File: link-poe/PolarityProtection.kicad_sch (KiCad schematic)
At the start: 6 parts, among them Q301 BSC010N04LS, Q302 BSC010N04LS, U301 LM74502-Q1

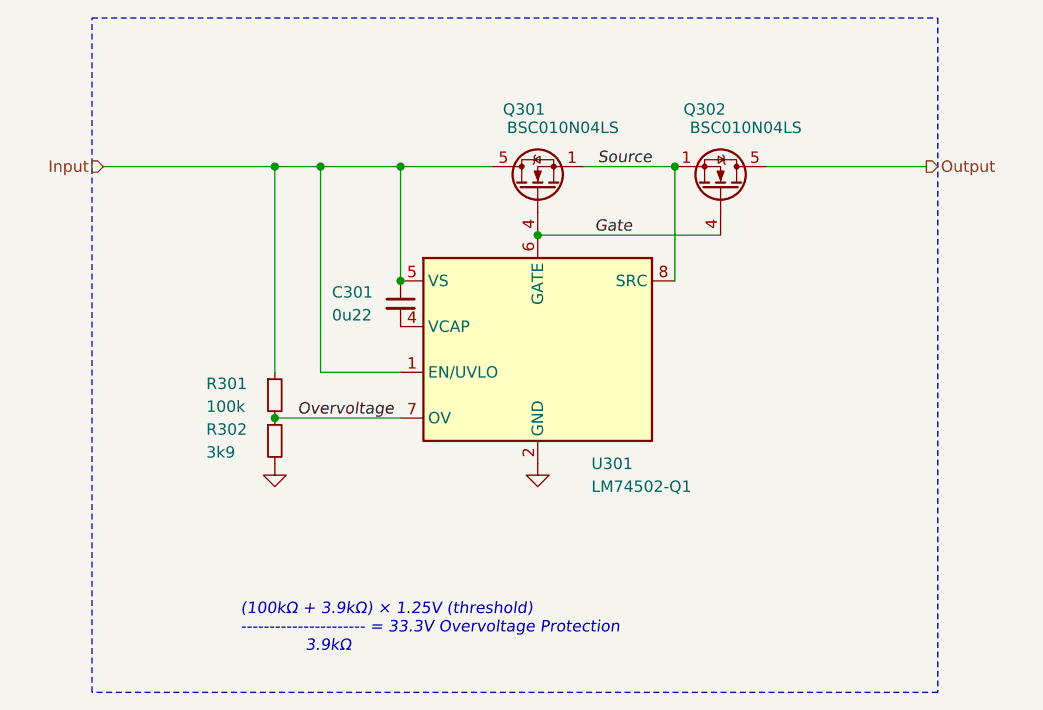
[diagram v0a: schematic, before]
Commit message: Update
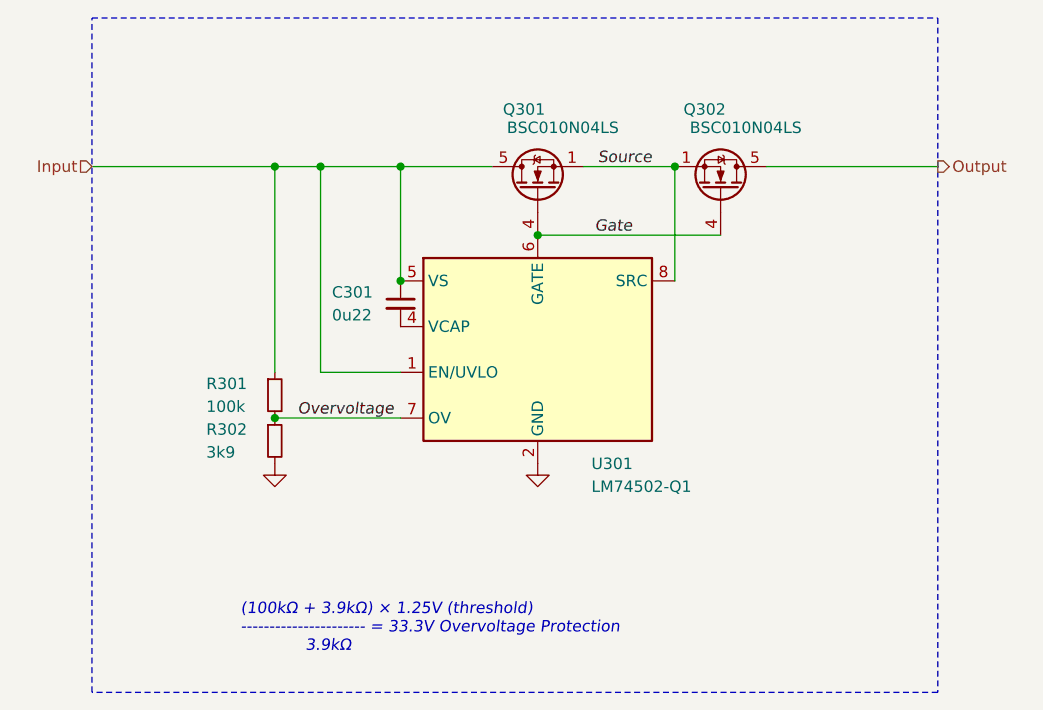
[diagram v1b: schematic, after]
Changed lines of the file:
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@@
 	(wire
 		(pts
-			(xy 102.87 86.36) (xy 121.92 86.36)
+			(xy 101.6 86.36) (xy 121.92 86.36)
 		)
 		(stroke
@@
 	(wire
 		(pts
-			(xy 176.53 86.36) (xy 194.31 86.36)
+			(xy 176.53 86.36) (xy 195.58 86.36)
 		)
 		(stroke
@@
 	(hierarchical_label "Input"
 		(shape input)
-		(at 102.87 86.36 180)
+		(at 101.6 86.36 180)
 		(effects
 			(font
@@
 	(hierarchical_label "Output"
 		(shape output)
-		(at 194.31 86.36 0)
+		(at 195.58 86.36 0)
 		(effects
 			(font

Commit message: Update usb + link-poe
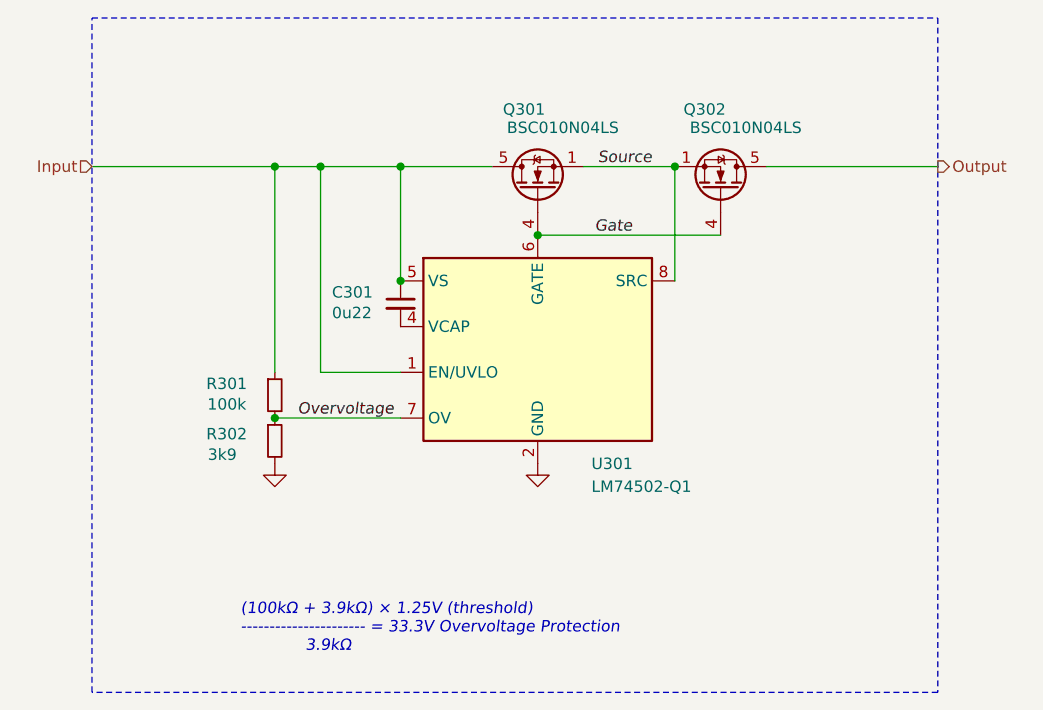
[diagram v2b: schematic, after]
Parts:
- C301: footprint Capacitor_SMD:C_0603_1608Metric -> V2_Capacitor_SMD:C_0603; symbol Device:C_Small -> V2_Device:C_0603_0u22; Mouser (none) -> 603-CC0603JRX79BB224
- Q301, Q302: Mouser (none) -> 726-BSC010N04LS
- R301: footprint Resistor_SMD:R_0603_1608Metric -> V2_Resistor_SMD:R_0603; symbol Device:R_Small -> V2_Device:R_0603_100k; Mouser (none) -> 71-CRCW0603100KFKEAC
- R302: footprint Resistor_SMD:R_0603_1608Metric -> V2_Resistor_SMD:R_0603; symbol Device:R_Small -> V2_Device:R_0603_3k9; Mouser (none) -> 71-CRCW06033K90FKEAC
- U301: Mouser (none) -> 595-LM74502HQDDFRQ1
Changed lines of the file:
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@@
+			)
+		)
+		(property "Mouser" "726-BSC010N04LS"
+			(at 166.878 88.9 0)
+			(effects
+				(font
+					(size 1.27 1.27)
+				)
+				(hide yes)
 			)
 		)
@@
 			)
 		)
+		(property "Mouser" "595-LM74502HQDDFRQ1"
+			(at 151.13 106.68 0)
+			(effects
+				(font
+					(size 1.27 1.27)
+				)
+				(hide yes)
+			)
+		)
 		(pin "1"
 		)
@@
 	)
 	(symbol
-		(lib_id "Device:R_Small")
+		(lib_id "V2_Device:R_0603_100k")
 		(at 121.92 111.76 0)
 		(unit 1)
@@
 		)
 		(property "Value" "100k"
-			(at 114.3 113.03 0)
-			(effects
-				(font
-					(size 1.27 1.27)
-				)
-				(justify left)
-			)
-		)
-		(property "Footprint" "Resistor_SMD:R_0603_1608Metric"
+			(at 116.586 112.776 0)
+			(effects
+				(font
+					(size 1.27 1.27)
+				)
+			)
+		)
+		(property "Footprint" "V2_Resistor_SMD:R_0603"
+			(at 121.92 127.508 0)
+			(effects
+				(font
+					(size 1.27 1.27)
+				)
+				(hide yes)
+			)
+		)
+		(property "Datasheet" ""
 			(at 121.92 111.76 0)
 			(effects
@@
 			)
 		)
-		(property "Datasheet" "~"
-			(at 121.92 111.76 0)
-			(effects
-				(font
-					(size 1.27 1.27)
-				)
-				(hide yes)
-			)
-		)
 		(property "Description" "Resistor, small symbol"
-			(at 121.92 111.76 0)
+			(at 121.92 123.952 0)
+			(effects
+				(font
+					(size 1.27 1.27)
+				)
+				(hide yes)
+			)
+		)
+		(property "Mouser" "71-CRCW0603100KFKEAC"
+			(at 121.92 127.254 0)
 			(effects
 				(font
@@
 	)
 	(symbol
-		(lib_id "Device:C_Small")
+		(lib_id "V2_Device:C_0603_0u22")
 		(at 135.89 101.6 0)
 		(unit 1)
@@
 		)
 		(property "Value" "0u22"
-			(at 128.27 102.87 0)
-			(effects
-				(font
-					(size 1.27 1.27)
-				)
-				(justify left)
-			)
-		)
-		(property "Footprint" "Capacitor_SMD:C_0603_1608Metric"
+			(at 128.27 102.616 0)
+			(effects
+				(font
+					(size 1.27 1.27)
+				)
+				(justify left)
+			)
+		)
+		(property "Footprint" "V2_Capacitor_SMD:C_0603"
+			(at 135.89 118.618 0)
+			(effects
+				(font
+					(size 1.27 1.27)
+				)
+				(hide yes)
+			)
+		)
+		(property "Datasheet" ""
 			(at 135.89 101.6 0)
 			(effects
@@
 			)
 		)
-		(property "Datasheet" "~"
-			(at 135.89 101.6 0)
-			(effects
-				(font
-					(size 1.27 1.27)
-				)
-				(hide yes)
-			)
-		)
 		(property "Description" "Unpolarized capacitor, small symbol"
-			(at 135.89 101.6 0)
+			(at 135.89 115.062 0)
+			(effects
+				(font
+					(size 1.27 1.27)
+				)
+				(hide yes)
+			)
+		)
+		(property "Mouser" "603-CC0603JRX79BB224"
+			(at 135.89 118.618 0)
 			(effects
 				(font
@@
 	)
 	(symbol
-		(lib_id "Device:R_Small")
+		(lib_id "V2_Device:R_0603_3k9")
 		(at 121.92 116.84 0)
 		(unit 1)
@@
 		(dnp no)
 		(property "Reference" "R302"
-			(at 114.3 115.57 0)
+			(at 114.3 116.078 0)
 			(effects
 				(font
@@
 		)
 		(property "Value" "3k9"
-			(at 114.3 118.11 0)
-			(effects
-				(font
-					(size 1.27 1.27)
-				)
-				(justify left)
-			)
-		)
-		(property "Footprint" "Resistor_SMD:R_0603_1608Metric"
+			(at 116.078 118.364 0)
+			(effects
+				(font
+					(size 1.27 1.27)
+				)
+			)
+		)
+		(property "Footprint" "V2_Resistor_SMD:R_0603"
+			(at 121.92 132.588 0)
+			(effects
+				(font
+					(size 1.27 1.27)
+				)
+				(hide yes)
+			)
+		)
+		(property "Datasheet" ""
 			(at 121.92 116.84 0)
 			(effects
@@
 			)
 		)
-		(property "Datasheet" "~"
-			(at 121.92 116.84 0)
-			(effects
-				(font
-					(size 1.27 1.27)
-				)
-				(hide yes)
-			)
-		)
 		(property "Description" "Resistor, small symbol"
-			(at 121.92 116.84 0)
+			(at 121.92 129.032 0)
+			(effects
+				(font
+					(size 1.27 1.27)
+				)
+				(hide yes)
+			)
+		)
+		(property "Mouser" "71-CRCW06033K90FKEAC"
+			(at 121.92 133.096 0)
 			(effects
 				(font
@@
 			(effects
 				(font
+					(size 1.27 1.27)
+				)
+				(hide yes)
+			)
+		)
+		(property "Mouser" "726-BSC010N04LS"
+			(at 155.702 88.9 0)
+			(effects
+				(font
